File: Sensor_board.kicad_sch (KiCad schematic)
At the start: 22 parts, among them U1001 LP5907MFX-1.8, U903 LP5907MFX-3.3

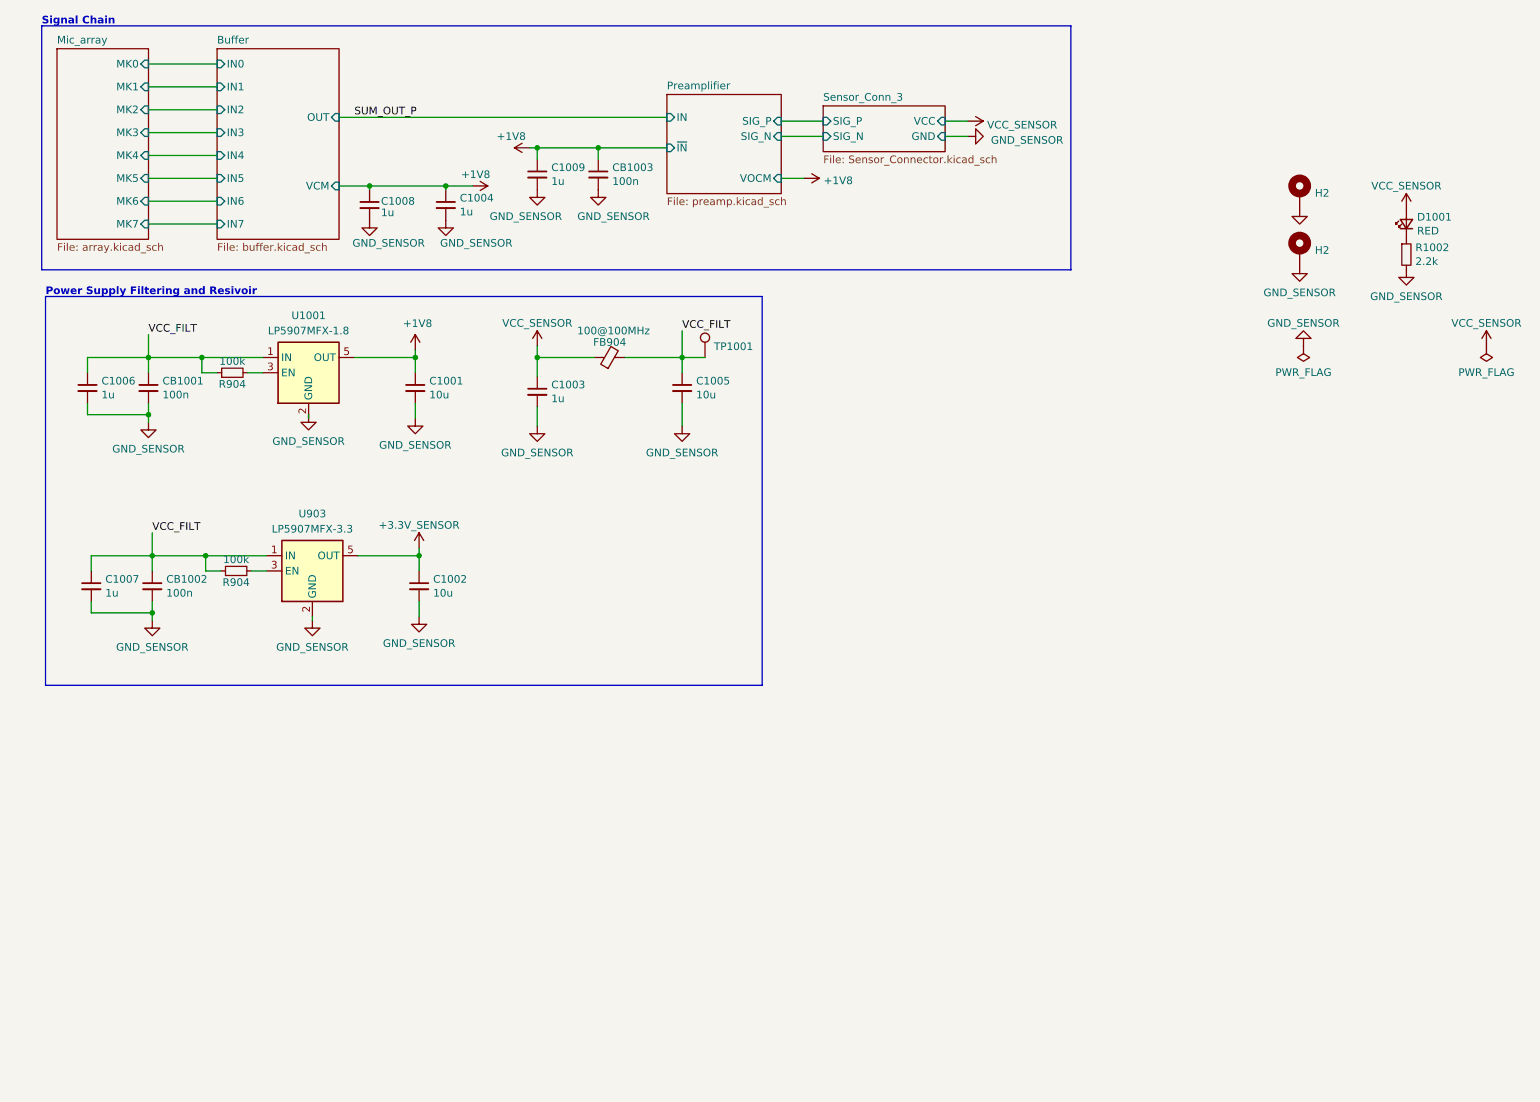
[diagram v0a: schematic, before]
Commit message: (sch) run DRC
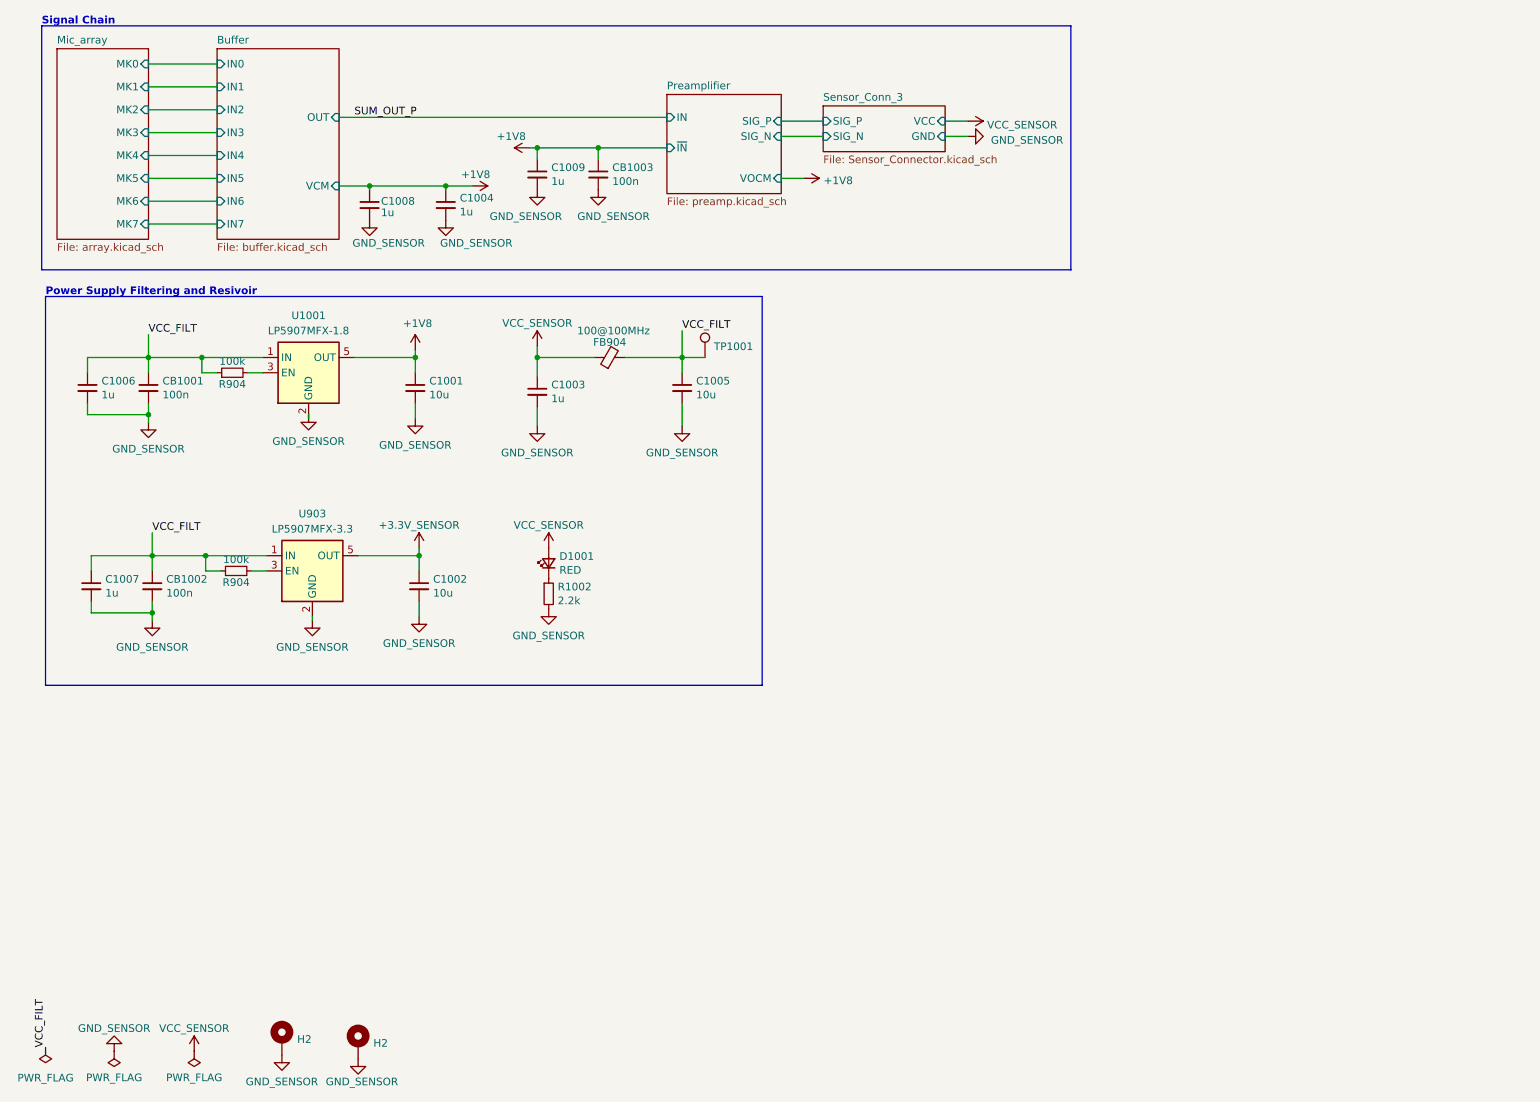
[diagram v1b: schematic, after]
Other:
- moved on the sheet: D1001, H2, R1002
